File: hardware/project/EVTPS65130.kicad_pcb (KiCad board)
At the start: 2 copper layers, 55 x 40 mm, 53 parts, among them J1 USB_C_Receptacle_PowerOnly_6P, J2 Conn_01x04_Pin, Q10 PMOS, U3 TPS65130RGE

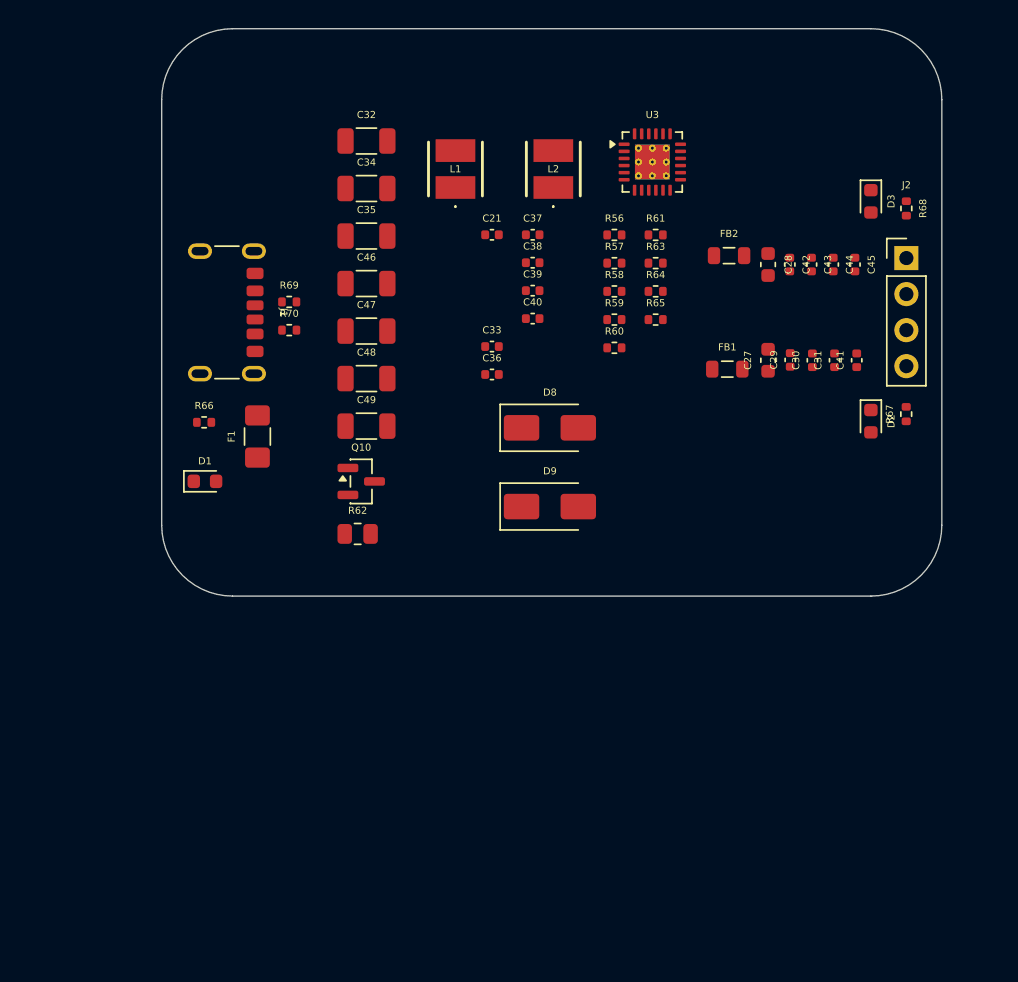
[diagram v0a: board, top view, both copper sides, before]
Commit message: Update
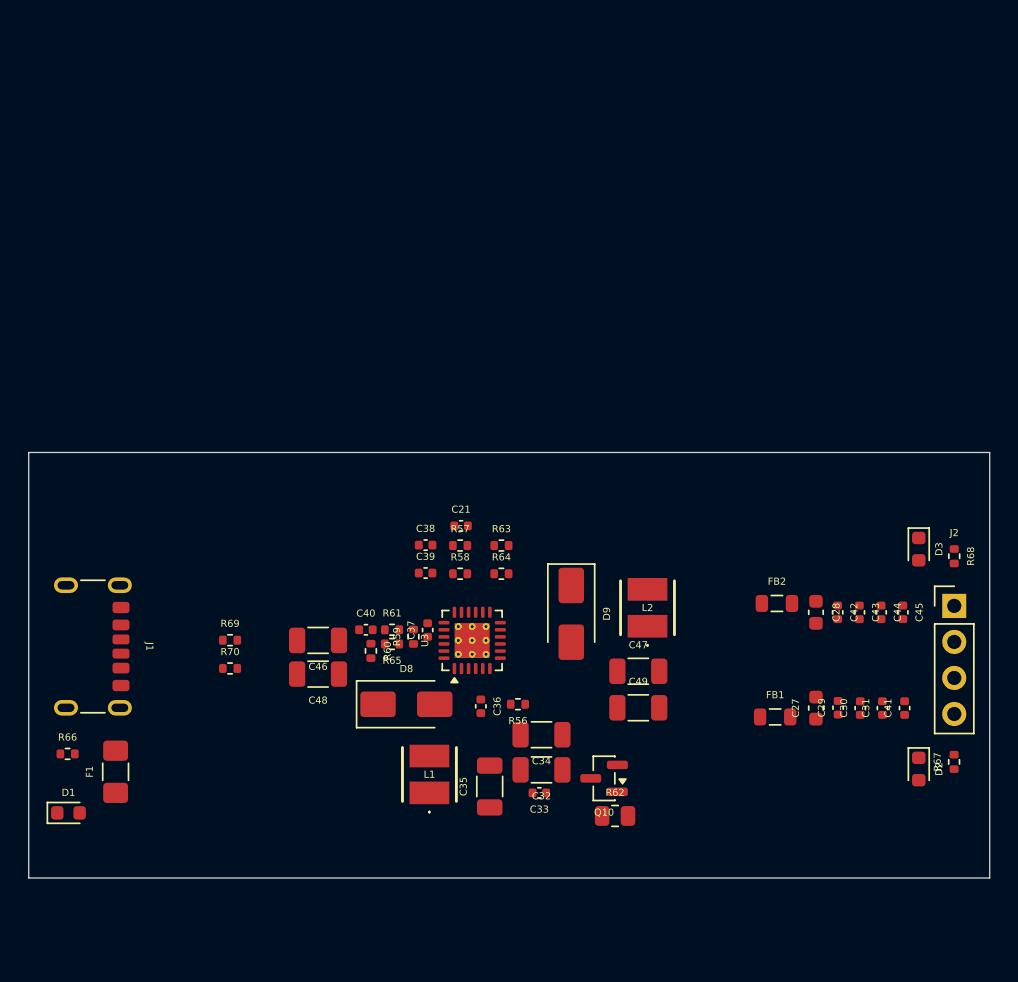
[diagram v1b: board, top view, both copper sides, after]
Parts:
- moved C32 46.0 mm to (149.3, 132.2), turned to 180 degrees
- moved L1 42.7 mm to (141.4, 132.6)
- moved C34 40.4 mm to (149.3, 129.8), turned to 180 degrees
- moved C35 39.8 mm to (145.6, 133.4), turned to 90 degrees
- moved U3 36.0 mm to (144.4, 123.1), turned to 90 degrees
- moved R56 33.8 mm to (147.6, 127.6), turned to 180 degrees
- moved R61 33.5 mm to (138.7, 122.4)
- moved C33 31.6 mm to (149.1, 133.9), turned to 180 degrees
- moved L2 31.6 mm to (156.8, 120.8)
- moved C47 30.7 mm to (156.1, 125.3)
- moved R65 29.5 mm to (138.7, 123.4), turned to 180 degrees
- moved C37 28.8 mm to (141.2, 122.4), turned to 90 degrees
- moved C49 27.6 mm to (156.1, 127.9)
- moved R60 27.4 mm to (137.2, 123.9), turned to -90 degrees
- moved Q10 27.0 mm to (153.7, 132.8), turned to 180 degrees
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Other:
- board size 55 x 40 mm -> 67.8 x 30 mm

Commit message: Updated PCB
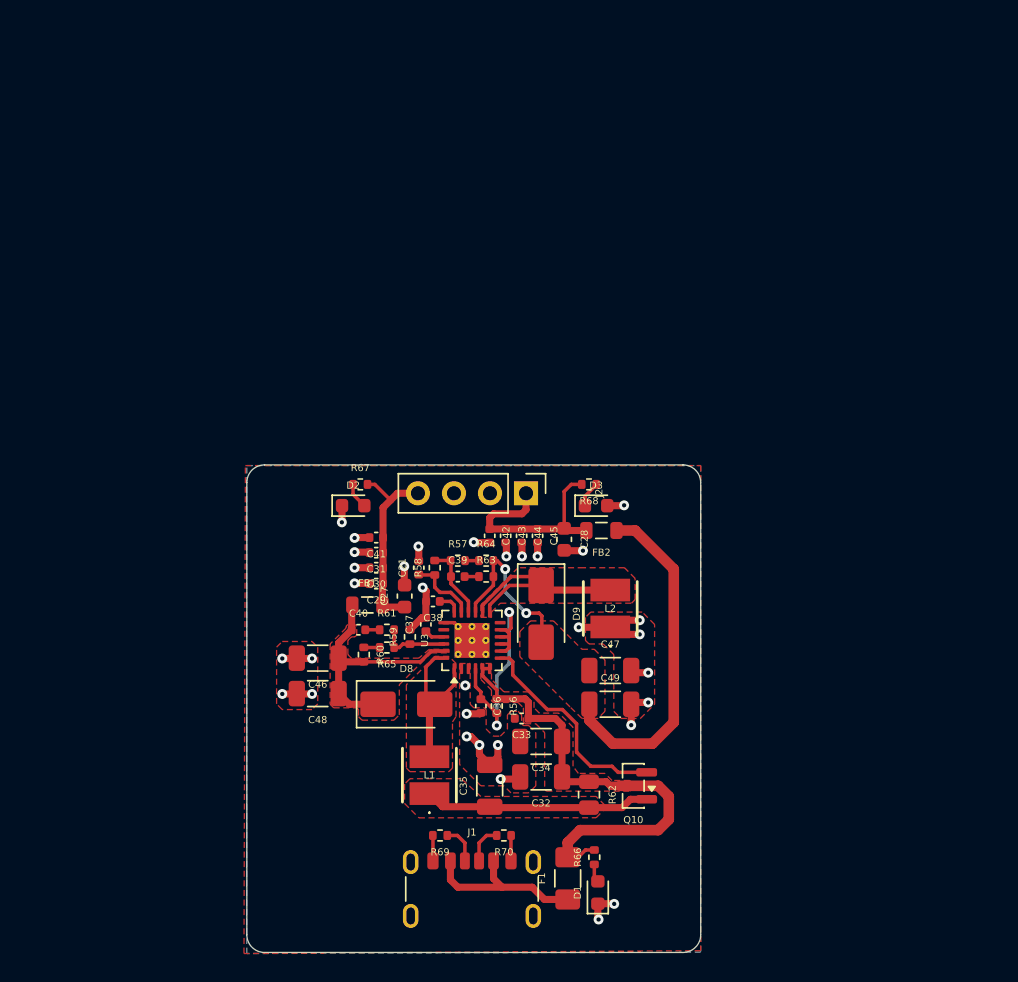
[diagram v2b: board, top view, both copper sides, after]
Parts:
- moved R67 46.2 mm to (136.5, 112.1), turned to 0 degrees
- moved D2 44.0 mm to (136.0, 113.6), turned to 0 degrees
- moved C41 39.1 mm to (137.6, 115.9), turned to 180 degrees
- moved R66 37.8 mm to (153.0, 138.4), turned to 90 degrees
- moved D1 37.7 mm to (153.2, 140.9), turned to 90 degrees
- moved C31 37.3 mm to (137.6, 116.9), turned to 180 degrees
- moved C30 35.5 mm to (137.6, 118.0), turned to 180 degrees
- moved C29 33.7 mm to (137.6, 119.1), turned to 180 degrees
- moved J1 33.2 mm to (144.4, 141.8), turned to 0 degrees
- moved F1 32.7 mm to (151.1, 139.9)
- moved J2 31.2 mm to (148.2, 112.8), turned to -90 degrees
- moved C27 30.1 mm to (139.6, 120.0)
- moved FB1 29.8 mm to (137.0, 120.6)
- moved C45 26.3 mm to (149.0, 115.8)
- moved R68 26.2 mm to (152.6, 112.1), turned to 180 degrees
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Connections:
- net Net-(D8-K) renamed /+12V_OUT
- net Net-(D9-A) renamed /-12V_OUT
- C27 pad 2: GND -> AGND
- C28 pad 2: GND -> AGND
- C29 pad 2: GND -> AGND
- C30 pad 2: GND -> AGND
- C31 pad 2: GND -> AGND
- C32 pad 2: GND -> AGND
- C33 pad 2: GND -> AGND
- C34 pad 2: GND -> AGND
- C35 pad 2: GND -> AGND
- C41 pad 2: GND -> AGND
- C42 pad 2: GND -> AGND
- C43 pad 2: GND -> AGND
- C44 pad 2: GND -> AGND
- C45 pad 2: GND -> AGND
- C46 pad 2: GND -> AGND
- C47 pad 2: GND -> AGND
- C48 pad 2: GND -> AGND
- C49 pad 2: GND -> AGND
- D1 pad 1: GND -> AGND
- D2 pad 1: GND -> AGND
- D3 pad 2: GND -> AGND
- J1 pad A12: GND -> AGND
- J1 pad B12: GND -> AGND
- J1 pad SH: GND -> AGND
- J2 pad 2: GND -> AGND
- J2 pad 3: GND -> AGND
- L2 pad 1: GND -> AGND
- R69 pad 2: GND -> AGND
- R70 pad 1: GND -> AGND
- U3 pad 2: GND -> AGND
- U3 pad 25: GND -> AGND
- U3 pad 3: GND -> AGND
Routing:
- net AGND: track 0.00 -> 47.2 mm, vias 0 -> 32
- net /-12V_OUT: track 0.00 -> 36.4 mm, vias 0 -> 2
- net VIN: track 0.00 -> 33.4 mm
- net Net-(U3-ENN): track 0.00 -> 18.4 mm, vias 0 -> 2
- net /+12V_OUT: track 0.00 -> 17.6 mm
- net Net-(Q10-D): track 0.00 -> 16.0 mm
- net VSS: track 0.00 -> 15.7 mm
- net Net-(D9-K): track 0.00 -> 15.4 mm
- net Net-(Q10-G): track 0.00 -> 15.4 mm
- net VDD: track 0.00 -> 13.5 mm
- net Net-(F1-Pad1): track 0.00 -> 12.3 mm
- net Net-(D8-A): track 0.02 -> 11.3 mm
- net Net-(U3-FBN): track 0.00 -> 5.28 mm
- net Net-(U3-VREF): track 0.00 -> 4.99 mm
- net Net-(U3-FBP): track 0.00 -> 4.86 mm
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- added copper zone on F.Cu, net /+12V_OUT
- added copper zone on F.Cu, net /-12V_OUT
- added copper zone on B.Cu, net AGND
- added copper zone on F.Cu, net AGND
- added copper zone on F.Cu, net Net-(D8-A)
- added copper zone on F.Cu, net Net-(D9-K)
- added copper zone on F.Cu, net Net-(Q10-D)
- added copper zone on F.Cu, net VIN
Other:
- board size 67.8 x 30 mm -> 32 x 34.4 mm
